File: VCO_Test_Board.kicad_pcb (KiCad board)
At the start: 2 copper layers, 99.1 x 71.1 mm, 19 parts, among them J1 PCB.SMAFRA.HT, J2 PCB.SMAFRA.HT, J3 Tune Voltage Input, J4 VCC, Y1 MAX2607EUT+T

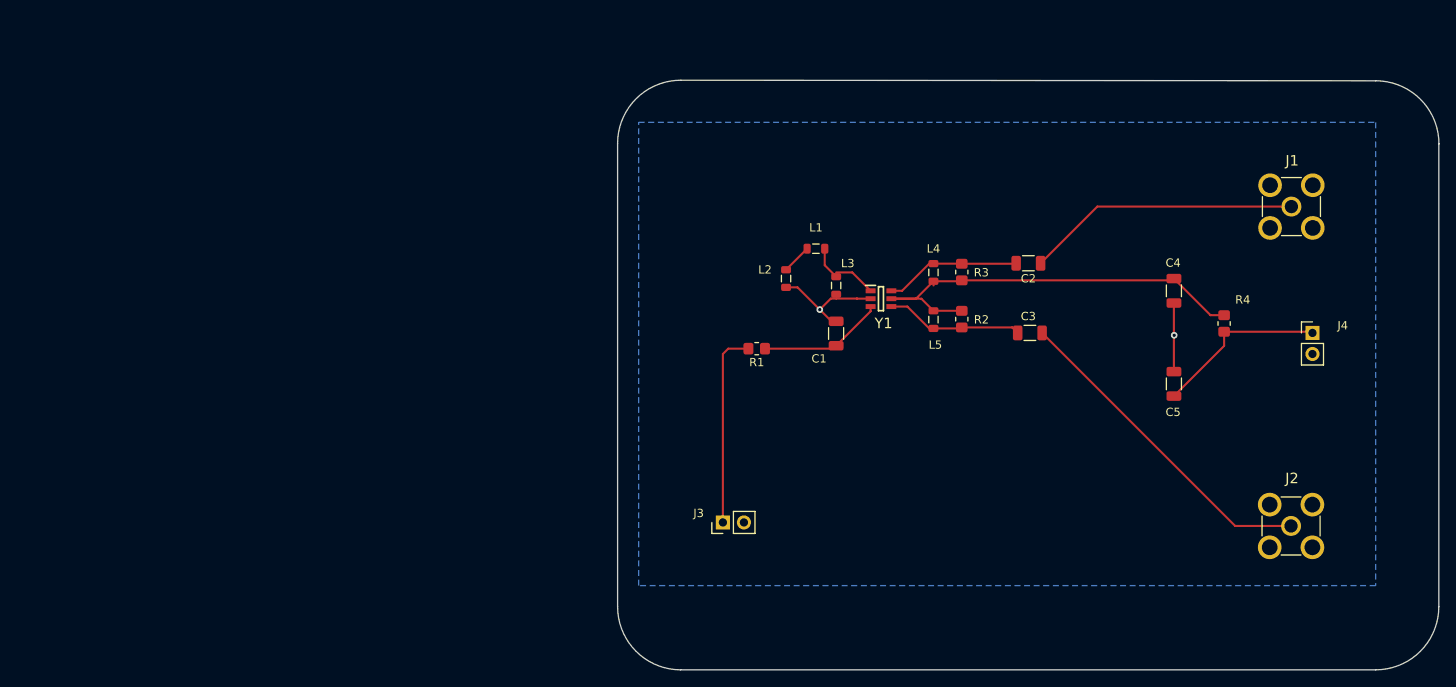
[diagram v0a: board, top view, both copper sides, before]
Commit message: Export gerber files.
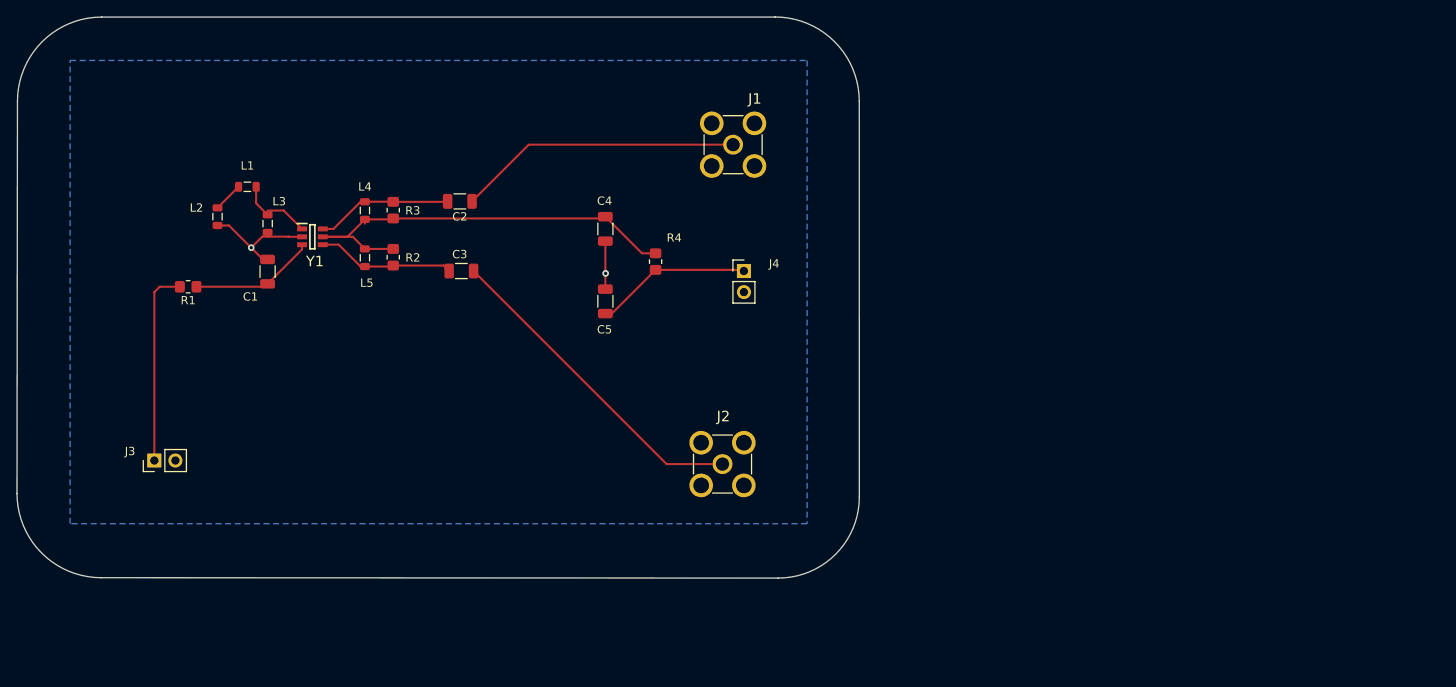
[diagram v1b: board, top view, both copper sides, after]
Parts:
- moved C5 69.3 mm to (95.0, 59.7)
- moved L2 69.0 mm to (48.3, 49.5)
- moved L3 69.0 mm to (54.3, 50.3)
- moved C1 69.0 mm to (54.3, 56.1)
- moved C3 69.0 mm to (77.7, 56.0)
- moved C4 69.0 mm to (95.0, 51.0)
- moved J2 69.0 mm to (109.2, 79.3)
- moved J3 69.0 mm to (40.6, 78.9)
- moved J4 69.0 mm to (111.8, 56.0)
- moved L1 69.0 mm to (51.9, 45.9)
- moved L4 69.0 mm to (66.0, 48.7)
- moved L5 69.0 mm to (66.0, 54.4)
- moved R1 69.0 mm to (44.7, 57.9)
- moved R2 69.0 mm to (69.5, 54.4)
- moved R3 69.0 mm to (69.5, 48.7)
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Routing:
- net GND: track 22.9 -> 20.4 mm
- net Net-(J4-Pin_1): track 21.0 -> 19.0 mm
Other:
- board size 99.1 x 71.1 mm -> 101.6 x 67.7 mm
